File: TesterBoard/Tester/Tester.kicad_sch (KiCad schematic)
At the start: 11 parts, among them Q1 LM7805CT_NOPB, U2 Z80CPU

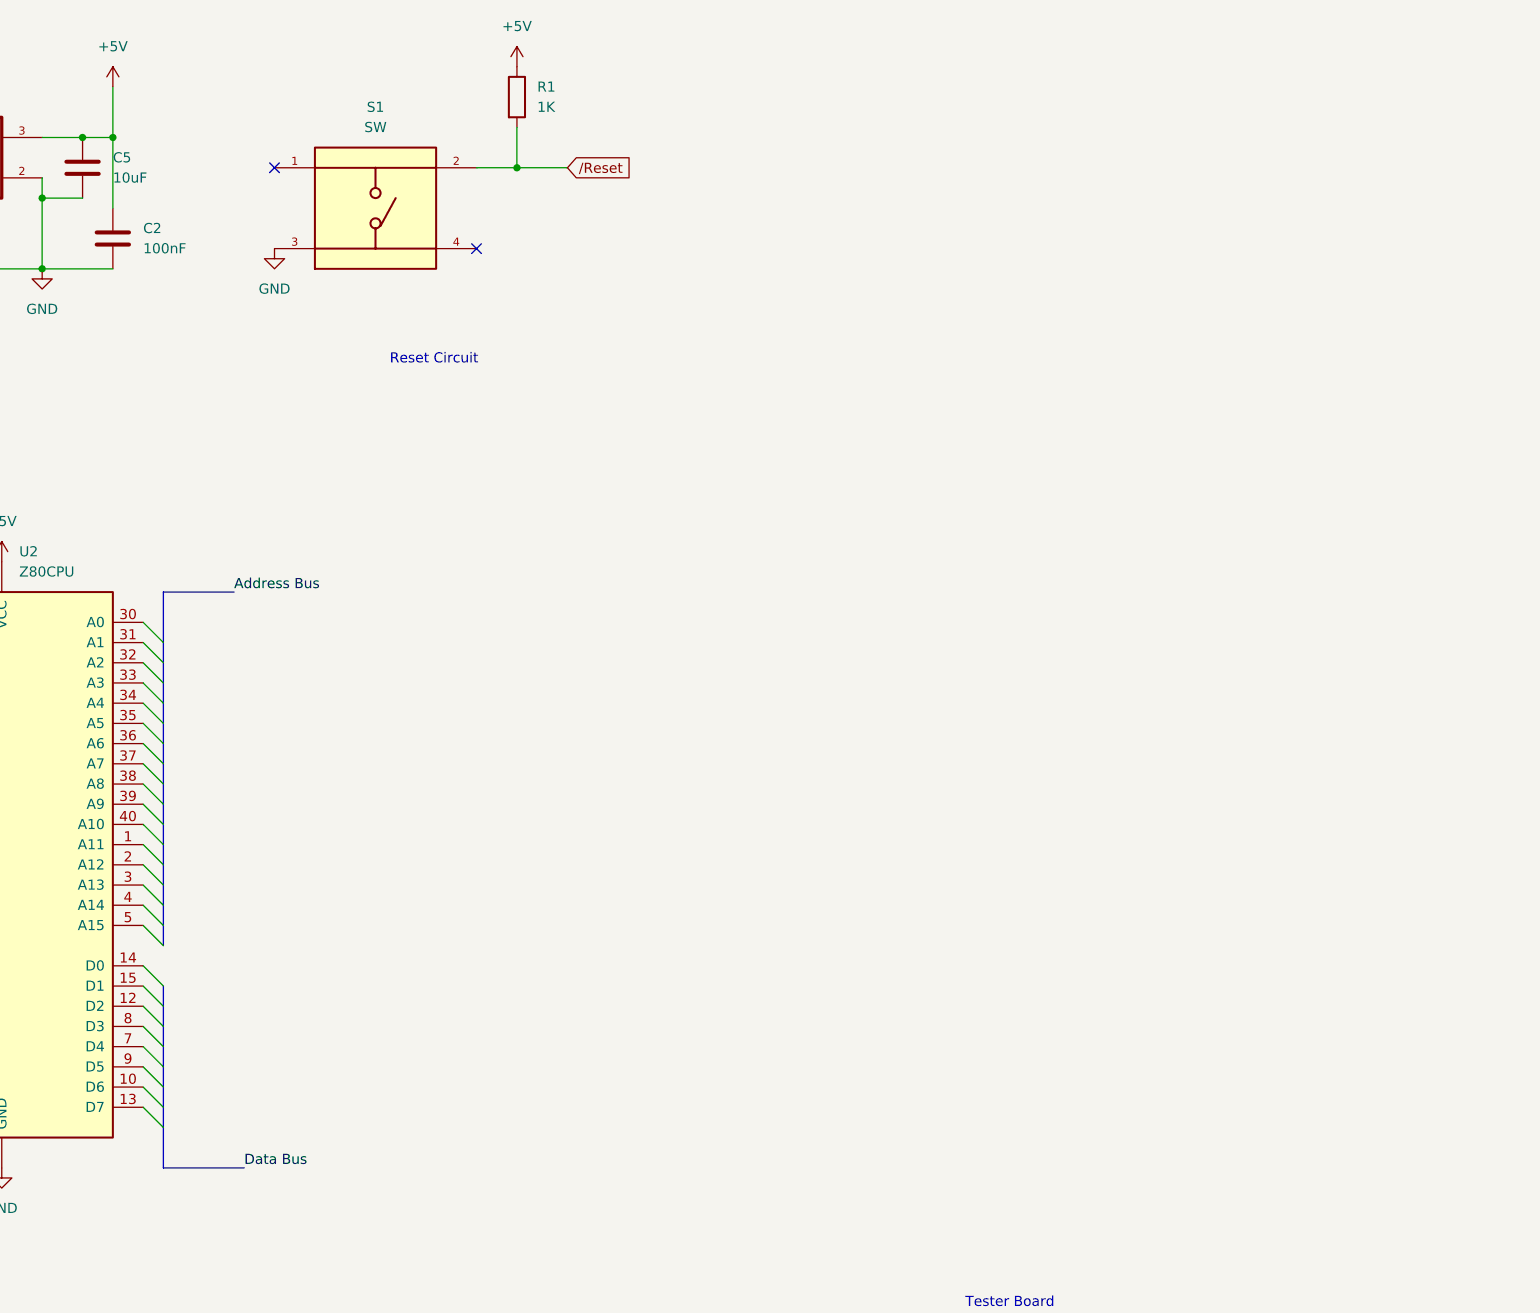
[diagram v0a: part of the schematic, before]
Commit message: pcb stuff
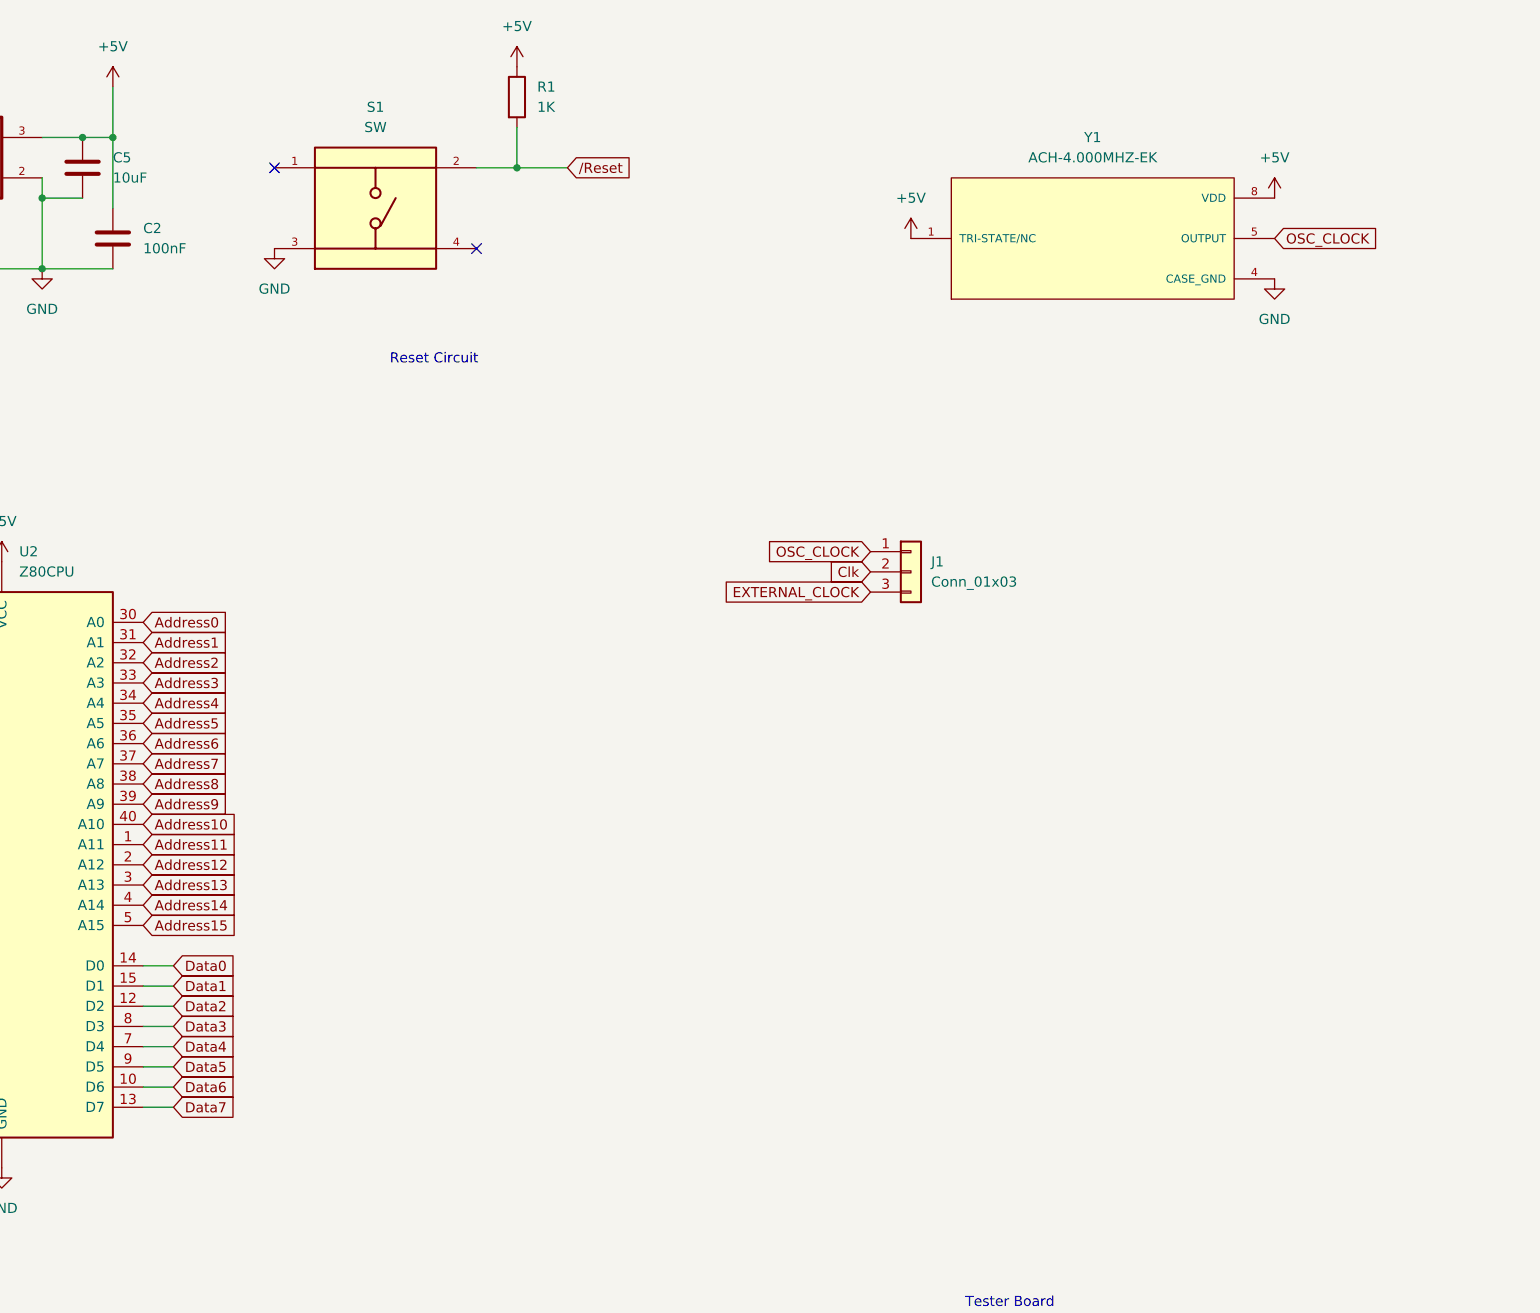
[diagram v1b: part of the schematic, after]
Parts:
- added J1: Conn_01x03, symbol Connector_Generic:Conn_01x03
- added Y1: ACH-4.000MHZ-EK, ACH-4.000MHZ-EK:XTAL_ACH-4.000MHZ-EK, symbol ACH-4.000MHZ-EK:ACH-4.000MHZ-EK
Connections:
- net +5V: now also Y1.1 (TRI-STATE/NC), Y1.8 (VDD)
- net Clk: now also J1.2 (Pin_2)
- net GND: now also Y1.4 (CASE_GND)
- net Address11: now reaches U2.1 (A11)
- net Data6: now reaches U2.10 (D6)
- net Data2: now reaches U2.12 (D2)
- net Data7: now reaches U2.13 (D7)
- net Data0: now reaches U2.14 (D0)
- net Data1: now reaches U2.15 (D1)
- net Address12: now reaches U2.2 (A12)
- net Address13: now reaches U2.3 (A13)
- net Address0: now reaches U2.30 (A0)
- net Address1: now reaches U2.31 (A1)
- net Address2: now reaches U2.32 (A2)
- net Address3: now reaches U2.33 (A3)
- net Address4: now reaches U2.34 (A4)
- net Address5: now reaches U2.35 (A5)
- net Address6: now reaches U2.36 (A6)
- net Address7: now reaches U2.37 (A7)
- net Address8: now reaches U2.38 (A8)
- net Address9: now reaches U2.39 (A9)
- net Address14: now reaches U2.4 (A14)
- net Address10: now reaches U2.40 (A10)
- net Address15: now reaches U2.5 (A15)
- net Data4: now reaches U2.7 (D4)
- net Data3: now reaches U2.8 (D3)
- net Data5: now reaches U2.9 (D5)
- new net EXTERNAL_CLOCK: J1.3 (Pin_3)
- new net OSC_CLOCK: J1.1 (Pin_1), Y1.5 (OUTPUT)
